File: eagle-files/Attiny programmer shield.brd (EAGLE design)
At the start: 68.6 x 53.3 mm, 16 parts, among them IC1 attiny10/11/12/13/15/22/25/45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, IC2 attiny24/44/84, IC3 attiny2313/4313

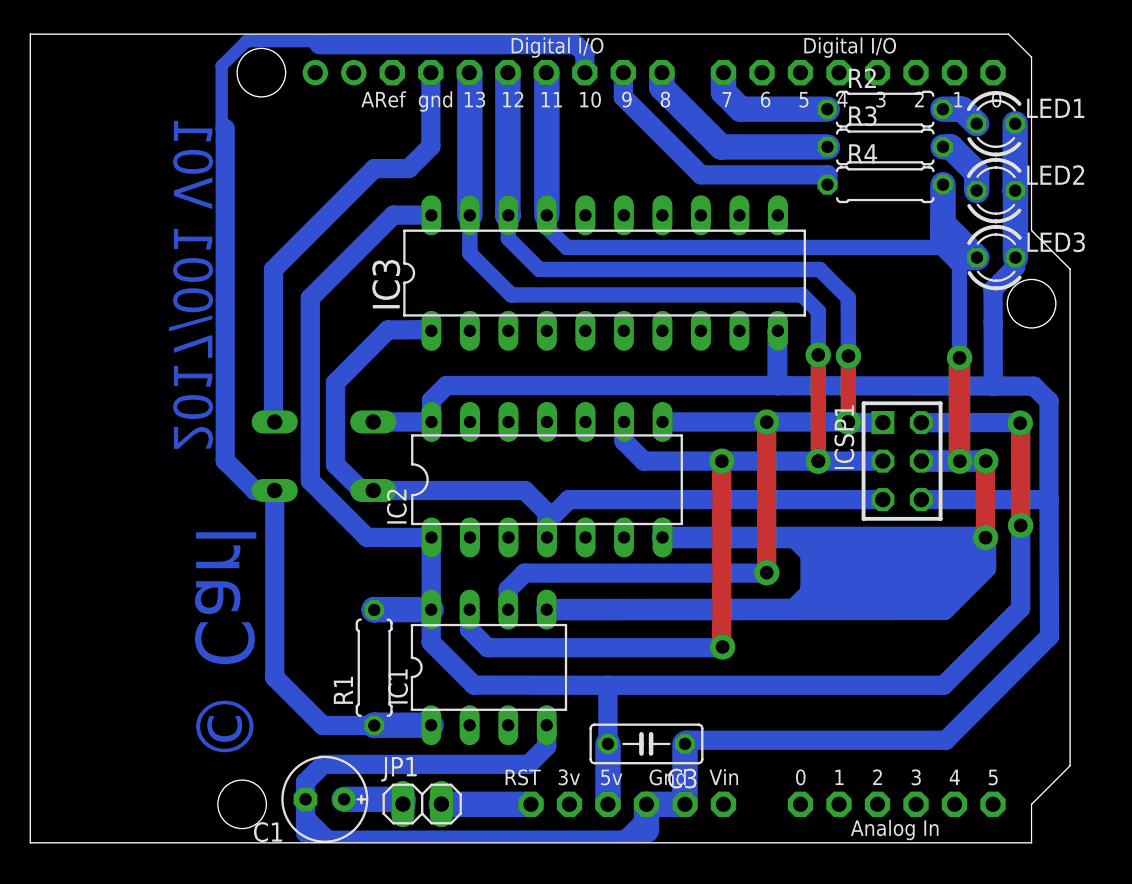
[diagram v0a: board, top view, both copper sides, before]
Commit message: .
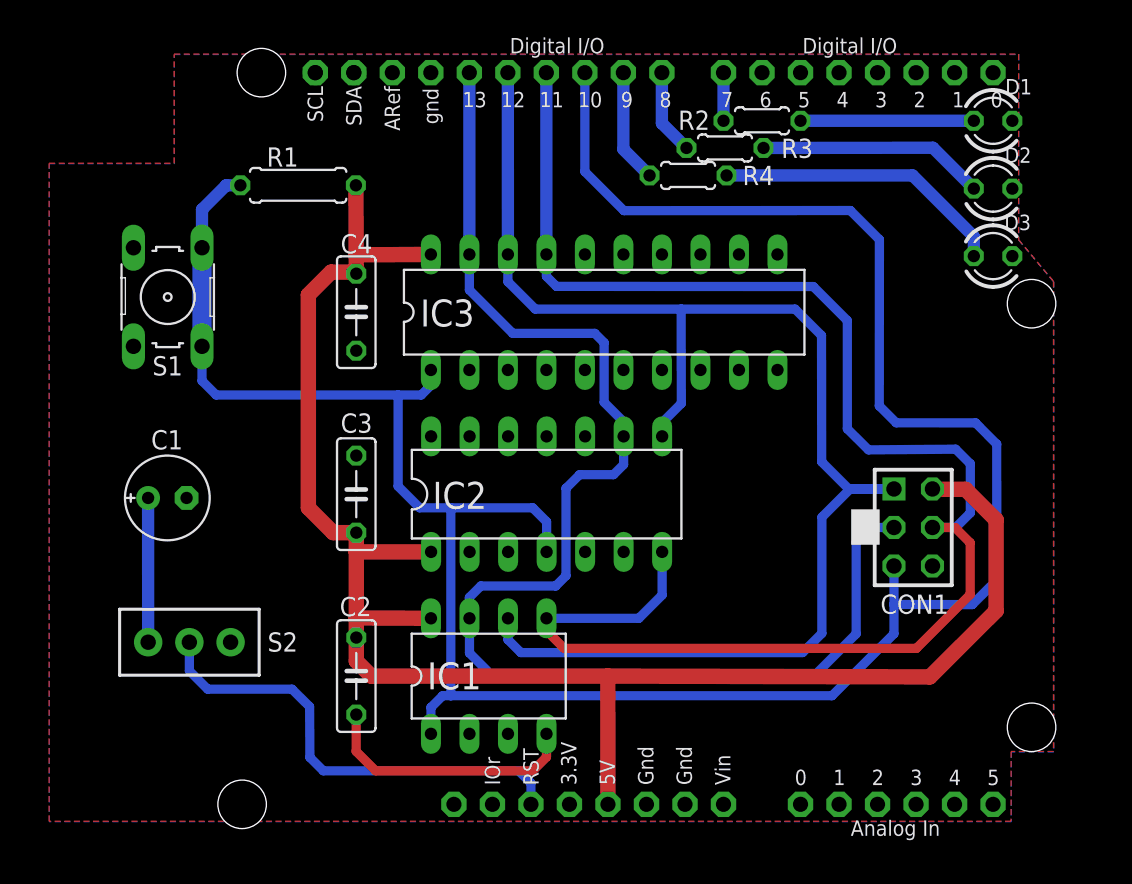
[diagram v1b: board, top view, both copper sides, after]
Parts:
- removed ICSP1: AVR-ISP-6, avr-4:AVR-ISP-6
- removed JP1: PROG-mode, pinhead:1X02
- removed LED1: Yellow - programming, led:LED3MM
- removed LED2: Red - error, led:LED3MM
- removed LED3: Green - ISP running, led:LED3MM
- added C2, C4: 100nF, rcl:C050-025X075
- added CON1: ICSP, avr-4:AVR-ISP-6
- added D1: Yellow - programming, led:LED3MM
- added D2: Red - error, led:LED3MM
- added D3: Green - ISP running, led:LED3MM
- added S2: prog-mode, ccr-lib:MINI_SPDT_SWITCH-9.0X4.0MM
- added U$2: (no value), base3clock:COPYRIGHT-LOGO-3-B
- added U$3: (no value), base3clock:3X-LOGO-10-B
- added U$4: (no value), base3clock:COPYRIGHT-LOGO-3-T
- added U$5: (no value), base3clock:3X-LOGO-5-B
- added U$6: (no value), base3clock:3X-LOGO-5-T
- R1: value 10kΩ -> 10k
- R2, R3, R4: value 270Ω -> 270; device resistor:0207/7 -> resistor:0204/5
- U$1: device adafruit:ARDUINO-BPLACE -> ccr-lib:ARDUINO-R3
- moved R1 32.2 mm to (17.7, 43.4), turned to 0 degrees
- moved C3 25.3 mm to (21.5, 23.0), turned to 270 degrees
- moved C1 22.4 mm to (9.04, 22.7), turned to 0 degrees
- moved S1 14.7 mm to (9.06, 36.0), flipped to the top, turned to 270 degrees
- moved R4 13.0 mm to (43.4, 44.0)
- moved R3 10.6 mm to (45.8, 45.8)
- moved R2 8.16 mm to (48.3, 47.6)
- moved IC3 2.58 mm to (37.9, 35.0)
- moved IC2 0.95 mm to (34.1, 23.0)
- moved IC1 0.57 mm to (30.2, 11.0)
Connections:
- net 3V renamed 3V3
- net +UB: now also C2.2, C4.2, CON1.2; no longer ICSP1.2
- net GND: now also C2.1, C4.1, CON1.6, D1.K, D2.K, D3.K; no longer ICSP1.6, LED1.K, LED2.K, LED3.K
- net MISO: now also CON1.1; no longer ICSP1.1
- net MOSI: now also CON1.4; no longer ICSP1.4
- net N$1: now also S2.3; no longer JP1.1
- net N$19: now also S2.2; no longer JP1.2
- net N$5: now also D1.A; no longer LED1.A
- net N$6: now also D2.A; no longer LED2.A
- net N$7: now also D3.A; no longer LED3.A
- net RESET: now also CON1.5; no longer ICSP1.5
- net SCK: now also CON1.3; no longer ICSP1.3
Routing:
- net GND: track 206.9 -> 17.4 mm
- net N$15: track 36.6 -> 0.00 mm
- net RESET: track 134.6 -> 165.2 mm
- net N$19: track 5.92 -> 30.8 mm
- net N$7: track 5.74 -> 19.3 mm
- net MOSI: track 116.8 -> 105.0 mm, vias 3 -> 0
- net N$6: track 4.10 -> 15.0 mm
- net N$2: track 17.9 -> 7.50 mm
- net N$5: track 2.63 -> 11.4 mm
- net SCK: track 98.8 -> 90.3 mm, vias 4 -> 0
- net MISO: track 86.6 -> 94.9 mm, vias 5 -> 0
- net N$4: track 13.5 -> 5.64 mm
- net N$3: track 8.60 -> 3.17 mm
- net N$1: track 4.19 -> 9.52 mm
- net N$13: track 4.57 -> 0.00 mm
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- added copper zone on layer 1, net GND
- added copper zone on layer 16, net GND
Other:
- board outline removed
- board text added: "2017/001 V02"
- board text added: "ATtiny 24/44/84"
- board text added: "ATtiny programmer shield"
- board text added: "ATtiny10/11/12/13/15 ATtiny22/25/45/85"
- board text added: "ATtiny2313 ATtiny4313"
- board text added: "Carl"
- board text added: "Designed by the Nostradomus Engineering Team"
- board text added: "Error!"
- board text added: "ISPrunning"
- board text added: "In Circuit System Programmer socket"
- board text added: "MISO"
- board text added: "MOSI"
- board text added: "PROG-RUN"
- board text added: "RESET"
- board text added: "SCK"
- board text added: "mode"
- board text added: "uploading"
- board text removed: "2017/001 V01"
- board text removed: "© Carl"
